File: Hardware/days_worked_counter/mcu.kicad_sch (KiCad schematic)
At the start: 16 parts, among them SW201 RESET, U201 ATmega328P-A, U202 DS1307Z+, Y201 16mhz, Y202 32.768kHz

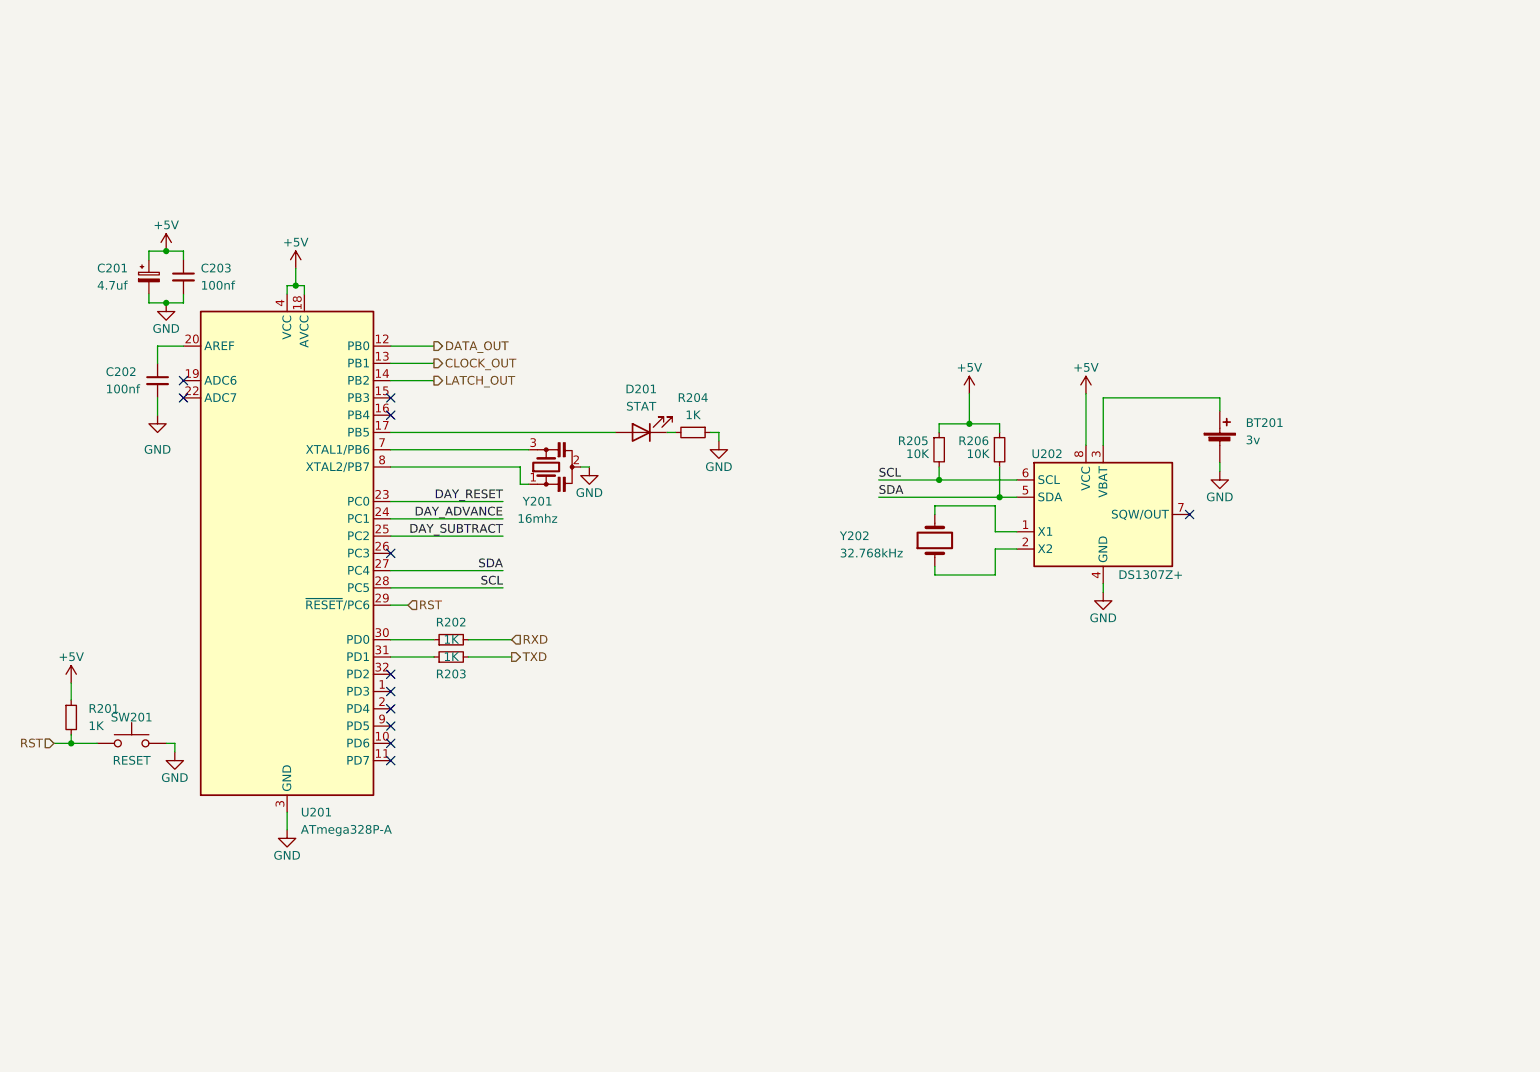
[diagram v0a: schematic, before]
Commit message: get input from @ka2qfx
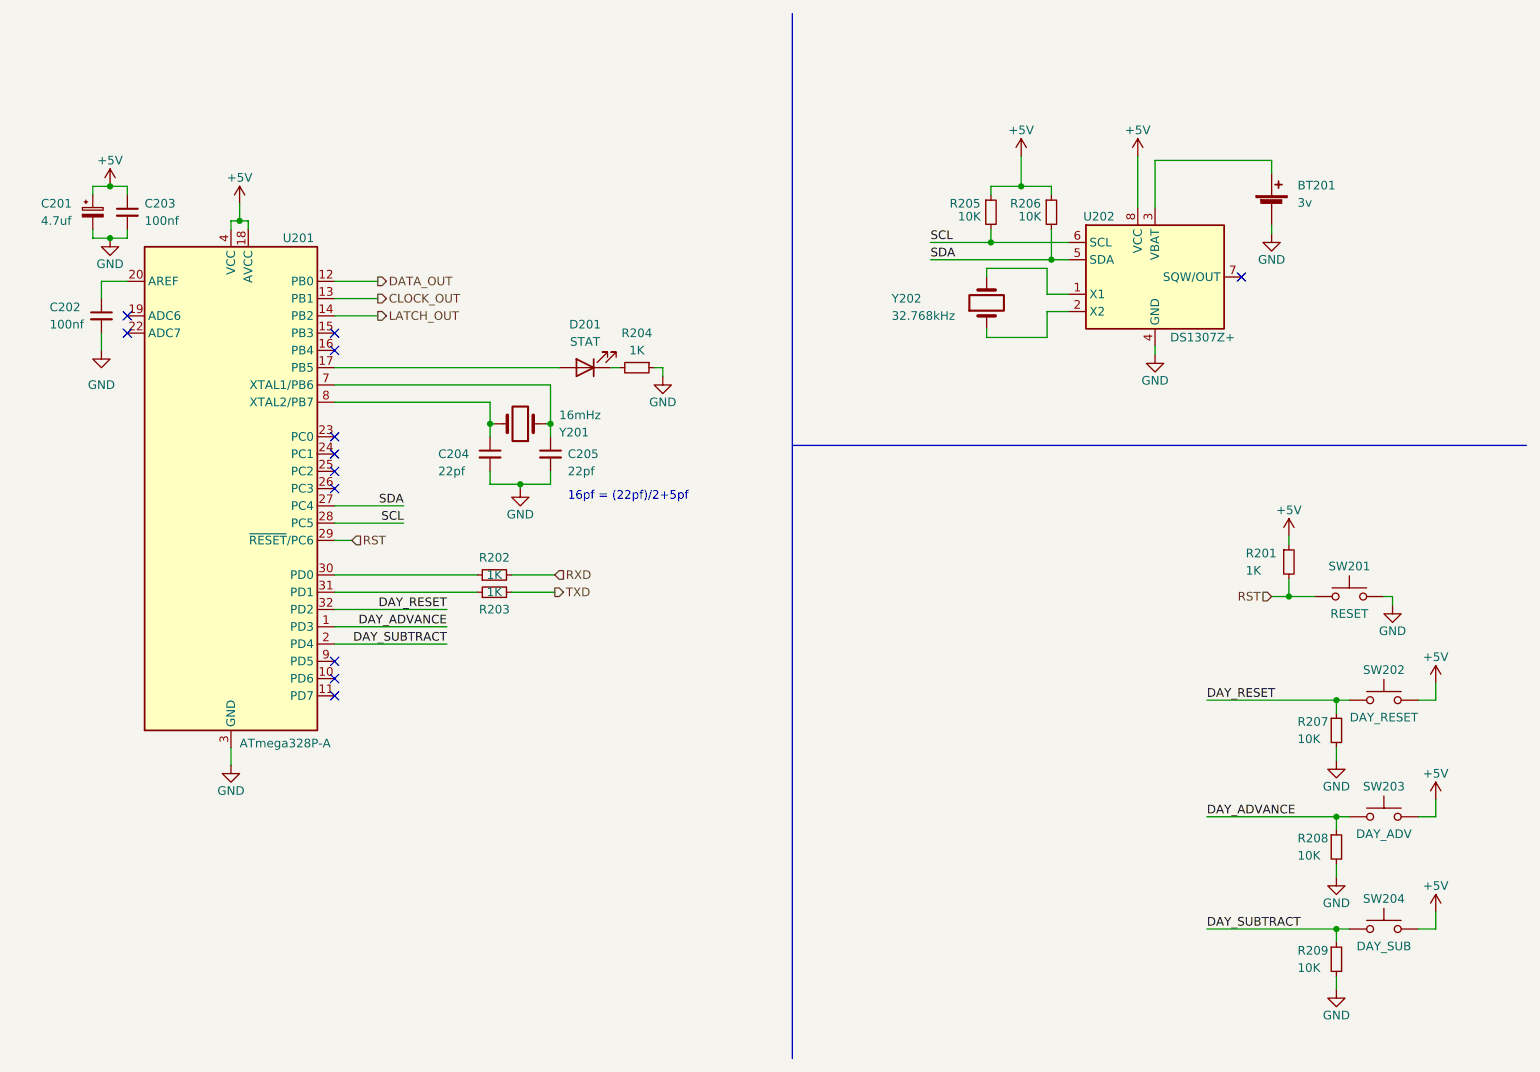
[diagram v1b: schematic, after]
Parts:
- removed Y201: 16mhz, symbol Device:Resonator_Small
- added C204, C205: 22pf, Capacitor_SMD:C_0805_2012Metric, symbol Device:C_Small
- added R207, R208, R209: 10K, Resistor_SMD:R_0805_2012Metric, symbol Device:R_Small
- added SW202: DAY_RESET, Button_Switch_THT:SW_PUSH_6mm_H5mm, symbol Switch:SW_Push
- added SW203: DAY_ADV, Button_Switch_THT:SW_PUSH_6mm_H5mm, symbol Switch:SW_Push
- added SW204: DAY_SUB, Button_Switch_THT:SW_PUSH_6mm_H5mm, symbol Switch:SW_Push
- added Y201: 16mHz, Crystal:Crystal_SMD_HC49-SD, symbol Device:Crystal
- SW201: footprint Button_Switch_SMD:SW_Push_SPST_NO_Alps_SKRK -> Button_Switch_THT:SW_PUSH_6mm_H5mm
- Y202: footprint (none) -> Crystal:Crystal_SMD_HC49-SD
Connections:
- net +5V: now also SW202.2, SW203.2, SW204.2
- net DAY_ADVANCE: now also U201.1 (PD3), R208.1, SW203.1; no longer U201.24 (PC1)
- net DAY_RESET: now also U201.32 (PD2), R207.1, SW202.1; no longer U201.23 (PC0)
- net DAY_SUBTRACT: now also U201.2 (PD4), R209.1, SW204.1; no longer U201.25 (PC2)
- net GND: now also C204.2, C205.2, R207.2, R208.2, R209.2
- net at U201.7 (XTAL1/PB6): now also C205.1, Y201.1
- net at U201.8 (XTAL2/PB7): now also C204.1, Y201.2
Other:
- note added: "16pf = (22pf)/2+5pf"
- moved on the sheet: BT201, C201, C202, C203, D201, R201, R202, R203, R204, R205, R206, SW201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
